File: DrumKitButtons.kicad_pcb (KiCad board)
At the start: 2 copper layers, 124.5 x 43.8 mm, 25 parts, among them J1 Input, J2 Output, U1 74HC165, U2 TLC5916

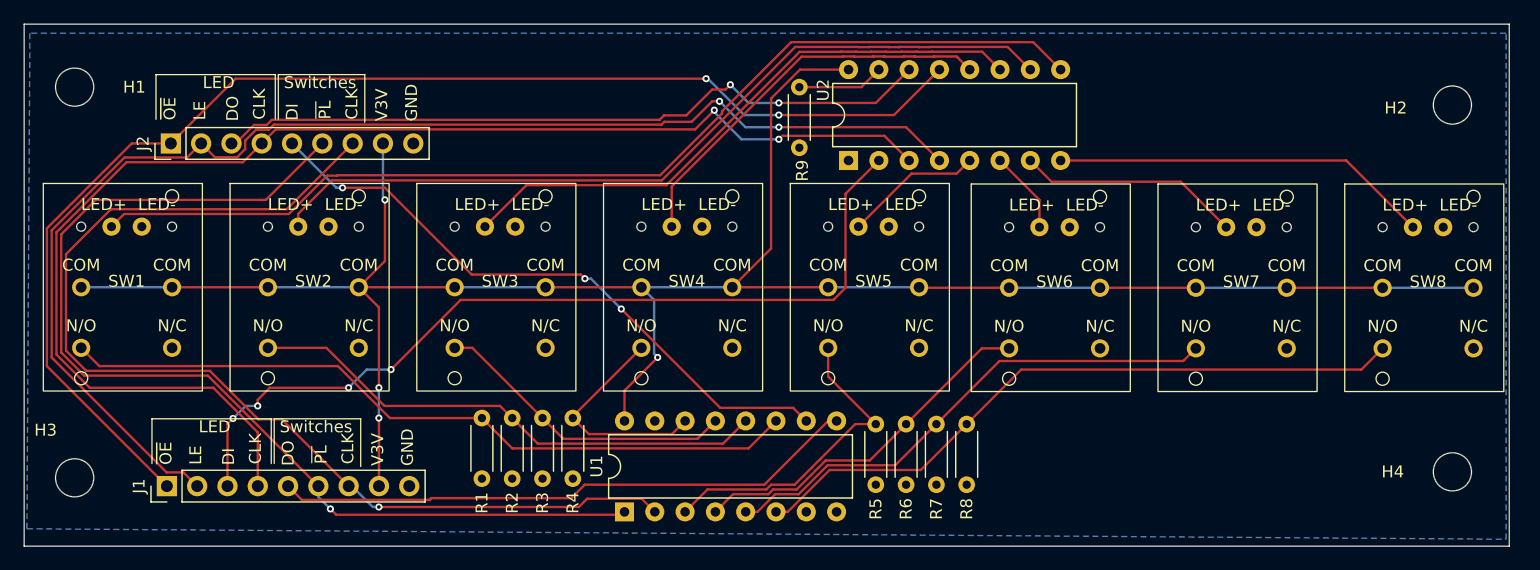
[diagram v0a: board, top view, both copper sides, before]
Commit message: next revision
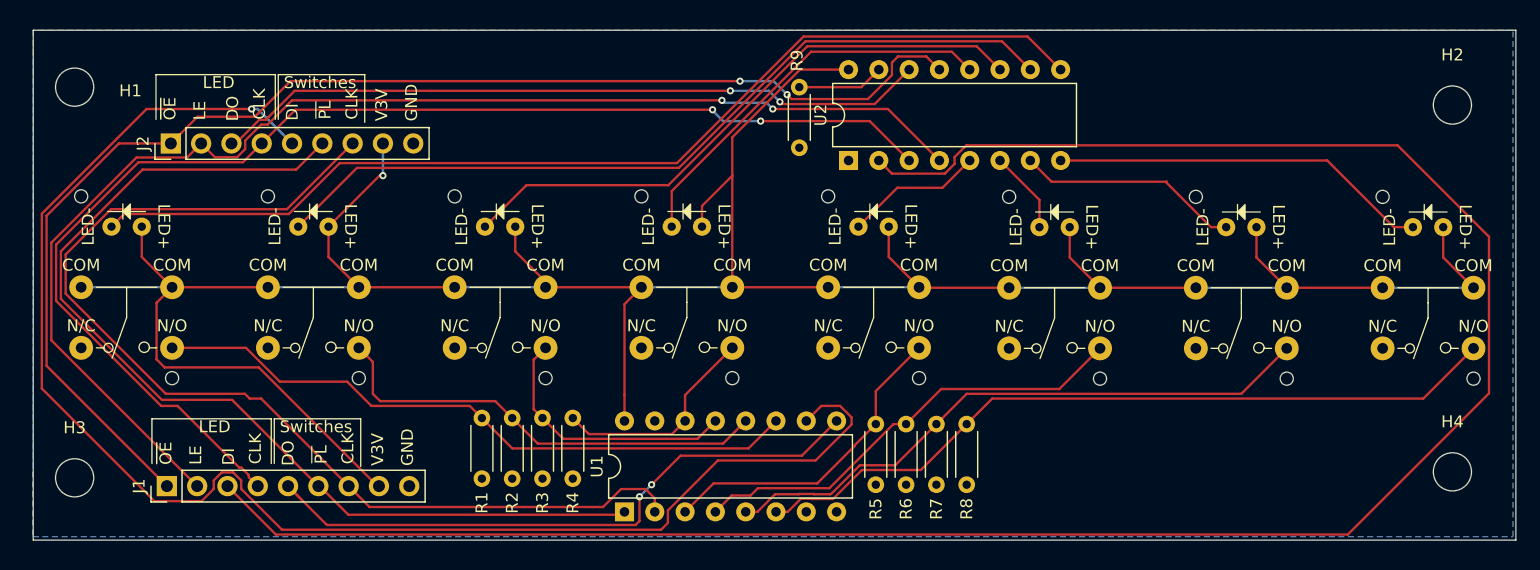
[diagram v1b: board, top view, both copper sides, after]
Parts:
- R9: value 250R -> 400R
- SW1, SW2, SW3, SW4, SW5, SW6, SW7, SW8: moved to B.Cu
- turned SW1 to 180 degrees
- turned SW2 to 180 degrees
- turned SW3 to 180 degrees
- turned SW4 to 180 degrees
- turned SW5 to 180 degrees
- turned SW6 to 180 degrees
- turned SW7 to 180 degrees
- turned SW8 to 180 degrees
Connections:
- SW1 pad 5: /LED_{1} -> VCC
- SW1 pad 6: GND -> /LED_{1}
- SW2 pad 5: /LED_{2} -> VCC
- SW2 pad 6: GND -> /LED_{2}
- SW3 pad 5: /LED_{3} -> VCC
- SW3 pad 6: GND -> /LED_{3}
- SW4 pad 5: /LED_{4} -> VCC
- SW4 pad 6: GND -> /LED_{4}
- SW5 pad 5: /LED_{5} -> VCC
- SW5 pad 6: GND -> /LED_{5}
- SW6 pad 5: /LED_{6} -> VCC
- SW6 pad 6: GND -> /LED_{6}
- SW7 pad 5: /LED_{7} -> VCC
- SW7 pad 6: GND -> /LED_{7}
- SW8 pad 5: /LED_{8} -> VCC
- SW8 pad 6: GND -> /LED_{8}
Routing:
- net /DI_{LED}: track 73.9 -> 181.6 mm, vias 4 -> 0
- net /DI_{SW}: track 52.7 -> 125.7 mm, vias 3 -> 1
- net VCC: track 185.2 -> 239.6 mm, vias 4 -> 1
- net /SW_{8}: track 56.5 -> 64.2 mm
- net /SW_{7}: track 43.4 -> 51.1 mm
- net /SW_{6}: track 30.3 -> 37.9 mm
- net /SW_{1}: track 62.7 -> 55.1 mm
- net /SW_{2}: track 44.2 -> 38.1 mm
- net /CLK_{LED}: track 112.1 -> 106.1 mm
- net /DO_{SW}: track 49.2 -> 53.8 mm, vias 0 -> 2
- net /~{PL_{SW}}: track 88.4 -> 84.2 mm, vias 1 -> 0
- net /SW_{3}: track 25.6 -> 22.4 mm
- net /LE_{LED}: track 110.1 -> 108.3 mm
- net /CLK_{SW}: track 91.5 -> 90.1 mm, vias 1 -> 0
- net /~{OE_{LED}}: track 108.6 -> 109.5 mm
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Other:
- board size 124.5 x 43.8 mm -> 124.3 x 42.7 mm
